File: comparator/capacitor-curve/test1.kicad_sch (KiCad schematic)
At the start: 3 parts

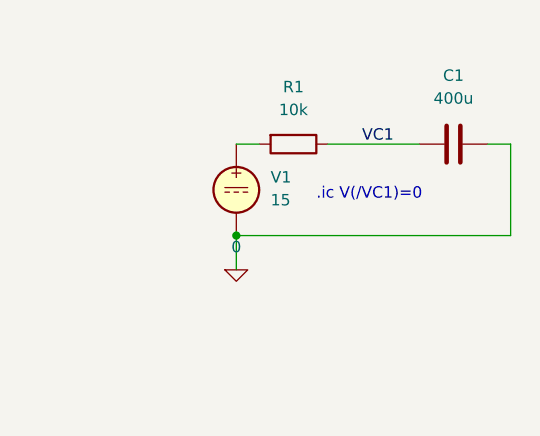
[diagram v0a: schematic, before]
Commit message: add/fix
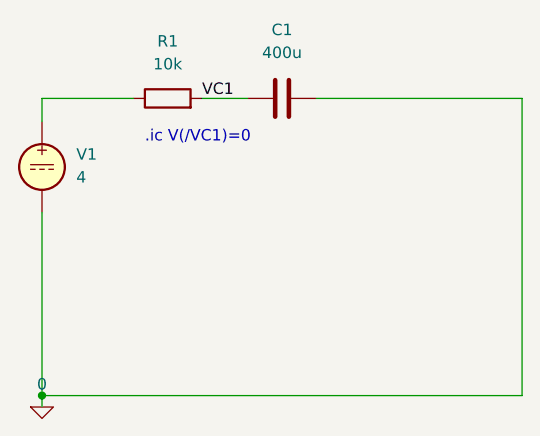
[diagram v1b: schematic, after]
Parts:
- V1: value 15 -> 4
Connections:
- net VC1: now also R1.2; no longer R1.1
- net at V1.1: now also R1.1; no longer R1.2
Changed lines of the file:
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@@
 (kicad_sch (version 20230121) (generator eeschema)
   (paper "A4")
-  (junction (at 81.28 90.17) (diameter 0) (color 0 0 0 0)
+  (junction (at 59.69 107.95) (diameter 0) (color 0 0 0 0)
   )
-  (wire (pts (xy 81.28 80.01) (xy 83.82 80.01))
+  (wire (pts (xy 113.03 107.95) (xy 113.03 74.93))
     (stroke (width 0) (type default))
   )
-  (wire (pts (xy 101.6 80.01) (xy 91.44 80.01))
+  (wire (pts (xy 59.69 109.22) (xy 59.69 107.95))
     (stroke (width 0) (type default))
   )
-  (wire (pts (xy 111.76 80.01) (xy 111.76 90.17))
+  (wire (pts (xy 59.69 77.47) (xy 59.69 74.93))
     (stroke (width 0) (type default))
   )
-  (wire (pts (xy 109.22 80.01) (xy 111.76 80.01))
+  (wire (pts (xy 90.17 74.93) (xy 113.03 74.93))
     (stroke (width 0) (type default))
   )
-  (wire (pts (xy 81.28 93.98) (xy 81.28 90.17))
+  (wire (pts (xy 59.69 87.63) (xy 59.69 107.95))
     (stroke (width 0) (type default))
   )
-  (wire (pts (xy 111.76 90.17) (xy 81.28 90.17))
+  (wire (pts (xy 59.69 74.93) (xy 69.85 74.93))
     (stroke (width 0) (type default))
   )
-  (text ".ic V(/VC1)=0" (at 90.17 86.36 0)
+  (wire (pts (xy 77.47 74.93) (xy 82.55 74.93))
+    (stroke (width 0) (type default))
+  )
+  (wire (pts (xy 59.69 107.95) (xy 113.03 107.95))
+    (stroke (width 0) (type default))
+  )
+  (text ".ic V(/VC1)=0" (at 71.12 80.01 0)
     (effects (font (size 1.27 1.27)) (justify left bottom))
   )
-  (label "VC1" (at 95.25 80.01 0) (fields_autoplaced)
+  (label "VC1" (at 77.47 74.93 0) (fields_autoplaced)
     (effects (font (size 1.27 1.27)) (justify left bottom))
   )
-  (symbol (lib_id "Simulation_SPICE:0") (at 81.28 93.98 0) (unit 1)
+  (symbol (lib_id "Simulation_SPICE:VDC") (at 59.69 82.55 0) (unit 1)
     (in_bom yes) (on_board yes) (dnp no) (fields_autoplaced)
-    (property "Reference" "#GND01" (at 81.28 96.52 0)
+    (property "Reference" "V1" (at 63.5 81.1502 0)
+      (effects (font (size 1.27 1.27)) (justify left))
+    )
+    (property "Value" "4" (at 63.5 83.6902 0)
+      (effects (font (size 1.27 1.27)) (justify left))
+    )
+    (property "Footprint" "" (at 59.69 82.55 0)
       (effects (font (size 1.27 1.27)) hide)
     )
-    (property "Value" "0" (at 81.28 91.44 0)
+    (property "Datasheet" "~" (at 59.69 82.55 0)
+      (effects (font (size 1.27 1.27)) hide)
+    )
+    (property "Sim.Pins" "1=+ 2=-" (at 59.69 82.55 0)
+      (effects (font (size 1.27 1.27)) hide)
+    )
+    (property "Sim.Type" "DC" (at 59.69 82.55 0)
+      (effects (font (size 1.27 1.27)) hide)
+    )
+    (property "Sim.Device" "V" (at 59.69 82.55 0)
+      (effects (font (size 1.27 1.27)) (justify left) hide)
+    )
+    (pin "1")
+    (pin "2")
+    (instances
+      (project "test1"
+        (path "/bb173b4d-9621-4ad4-b8d6-5552f010e489"
+          (reference "V1") (unit 1)
+        )
+      )
+    )
+  )
+  (symbol (lib_id "Device:C") (at 86.36 74.93 90) (unit 1)
+    (in_bom yes) (on_board yes) (dnp no) (fields_autoplaced)
+    (property "Reference" "C1" (at 86.36 67.31 90)
       (effects (font (size 1.27 1.27)))
     )
-    (property "Footprint" "" (at 81.28 93.98 0)
+    (property "Value" "400u" (at 86.36 69.85 90)
+      (effects (font (size 1.27 1.27)))
+    )
+    (property "Footprint" "" (at 90.17 73.9648 0)
       (effects (font (size 1.27 1.27)) hide)
     )
-    (property "Datasheet" "~" (at 81.28 93.98 0)
+    (property "Datasheet" "~" (at 86.36 74.93 0)
+      (effects (font (size 1.27 1.27)) hide)
+    )
+    (pin "1")
+    (pin "2")
+    (instances
+      (project "test1"
+        (path "/bb173b4d-9621-4ad4-b8d6-5552f010e489"
+          (reference "C1") (unit 1)
+        )
+      )
+    )
+  )
+  (symbol (lib_id "Simulation_SPICE:0") (at 59.69 109.22 0) (unit 1)
+    (in_bom yes) (on_board yes) (dnp no) (fields_autoplaced)
+    (property "Reference" "#GND01" (at 59.69 111.76 0)
+      (effects (font (size 1.27 1.27)) hide)
+    )
+    (property "Value" "0" (at 59.69 106.68 0)
+      (effects (font (size 1.27 1.27)))
+    )
+    (property "Footprint" "" (at 59.69 109.22 0)
+      (effects (font (size 1.27 1.27)) hide)
+    )
+    (property "Datasheet" "~" (at 59.69 109.22 0)
       (effects (font (size 1.27 1.27)) hide)
     )
     (pin "1")
     (instances
-      (project "test-details"
-        (path "/8300bb89-af22-40bb-96f5-ff500b49d277"
+      (project "test1"
+        (path "/bb173b4d-9621-4ad4-b8d6-5552f010e489"
           (reference "#GND01") (unit 1)
         )
@@
     )
   )
-  (symbol (lib_id "Simulation_SPICE:VDC") (at 81.28 85.09 0) (unit 1)
+  (symbol (lib_id "Device:R") (at 73.66 74.93 90) (unit 1)
     (in_bom yes) (on_board yes) (dnp no) (fields_autoplaced)
-    (property "Reference" "V1" (at 85.09 83.6902 0)
-      (effects (font (size 1.27 1.27)) (justify left))
+    (property "Reference" "R1" (at 73.66 68.58 90)
+      (effects (font (size 1.27 1.27)))
     )
-    (property "Value" "15" (at 85.09 86.2302 0)
-      (effects (font (size 1.27 1.27)) (justify left))
+    (property "Value" "10k" (at 73.66 71.12 90)
+      (effects (font (size 1.27 1.27)))
     )
-    (property "Footprint" "" (at 81.28 85.09 0)
+    (property "Footprint" "" (at 73.66 76.708 90)
       (effects (font (size 1.27 1.27)) hide)
     )
-    (property "Datasheet" "~" (at 81.28 85.09 0)
-      (effects (font (size 1.27 1.27)) hide)
-    )
-    (property "Sim.Pins" "1=+ 2=-" (at 81.28 85.09 0)
-      (effects (font (size 1.27 1.27)) hide)
-    )
-    (property "Sim.Type" "DC" (at 81.28 85.09 0)
-      (effects (font (size 1.27 1.27)) hide)
-    )
-    (property "Sim.Device" "V" (at 81.28 85.09 0)
-      (effects (font (size 1.27 1.27)) (justify left) hide)
-    )
-    (pin "1")
-    (pin "2")
-    (instances
-      (project "test-details"
-        (path "/8300bb89-af22-40bb-96f5-ff500b49d277"
-          (reference "V1") (unit 1)
-        )
-      )
-    )
-  )
-  (symbol (lib_id "Device:C") (at 105.41 80.01 90) (unit 1)
-    (in_bom yes) (on_board yes) (dnp no) (fields_autoplaced)
-    (property "Reference" "C1" (at 105.41 72.39 90)
-      (effects (font (size 1.27 1.27)))
-    )
-    (property "Value" "400u" (at 105.41 74.93 90)
-      (effects (font (size 1.27 1.27)))
-    )
-    (property "Footprint" "" (at 109.22 79.0448 0)
-      (effects (font (size 1.27 1.27)) hide)
-    )
-    (property "Datasheet" "~" (at 105.41 80.01 0)
+    (property "Datasheet" "~" (at 73.66 74.93 0)
       (effects (font (size 1.27 1.27)) hide)
     )
@@
     (pin "2")
     (instances
-      (project "test-details"
-        (path "/8300bb89-af22-40bb-96f5-ff500b49d277"
-          (reference "C1") (unit 1)
-        )
-      )
-    )
-  )
-  (symbol (lib_id "Device:R") (at 87.63 80.01 270) (unit 1)
-    (in_bom yes) (on_board yes) (dnp no) (fields_autoplaced)
-    (property "Reference" "R1" (at 87.63 73.66 90)
-      (effects (font (size 1.27 1.27)))
-    )
-    (property "Value" "10k" (at 87.63 76.2 90)
-      (effects (font (size 1.27 1.27)))
-    )
-    (property "Footprint" "" (at 87.63 78.232 90)
-      (effects (font (size 1.27 1.27)) hide)
-    )
-    (property "Datasheet" "~" (at 87.63 80.01 0)
-      (effects (font (size 1.27 1.27)) hide)
-    )
-    (pin "1")
-    (pin "2")
-    (instances
-      (project "test-details"
-        (path "/8300bb89-af22-40bb-96f5-ff500b49d277"
+      (project "test1"
+        (path "/bb173b4d-9621-4ad4-b8d6-5552f010e489"
           (reference "R1") (unit 1)
         )
